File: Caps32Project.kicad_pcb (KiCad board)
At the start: 2 copper layers, 20 x 33 mm, 36 parts, among them J1 Ph 2.0, J2 Sh 1.0, P1 USB_C_Plug_USB2.0, Q1 AO3401A, U1 MPU-6050, U2 IP5306, U3 ESP32C3_SuperMini

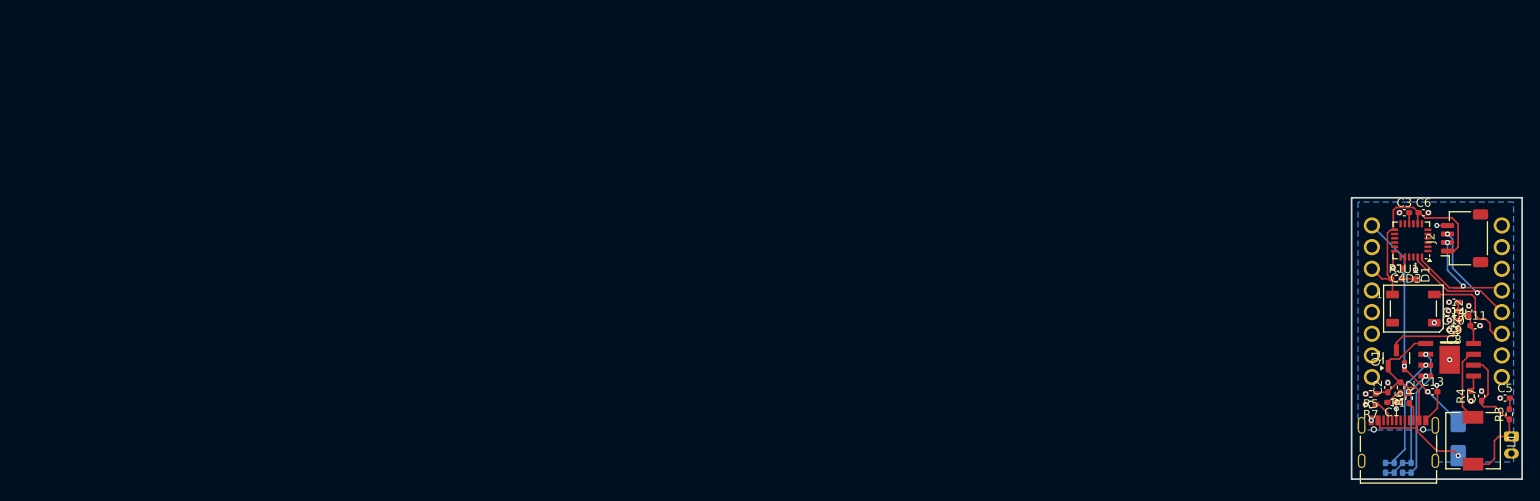
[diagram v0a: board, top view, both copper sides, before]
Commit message: Tweak
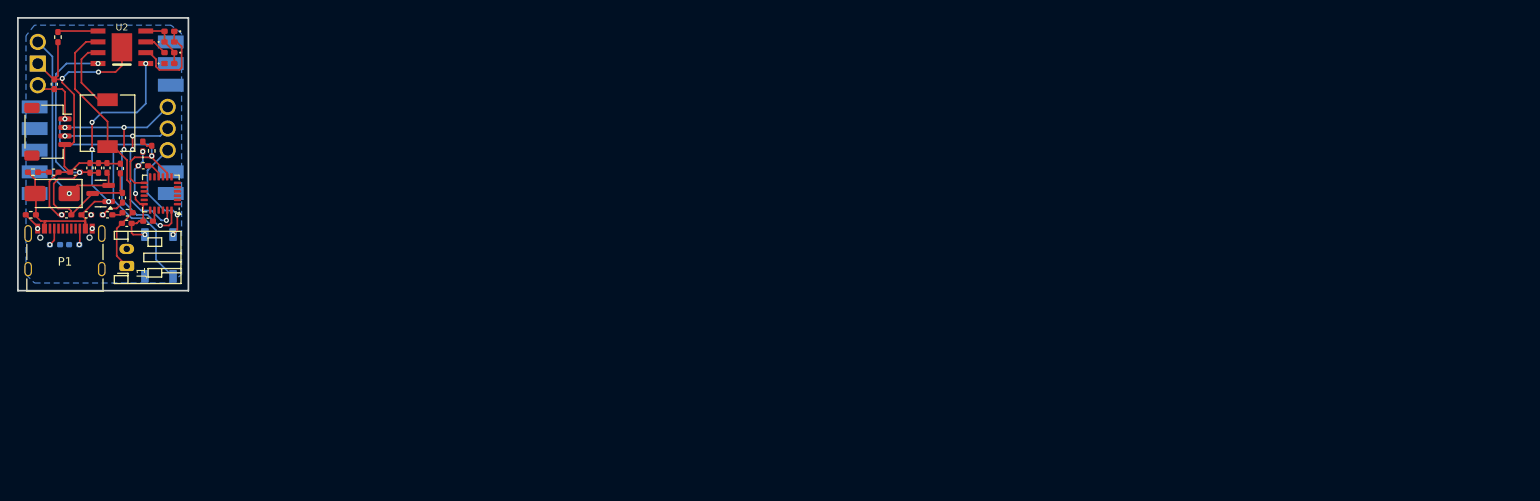
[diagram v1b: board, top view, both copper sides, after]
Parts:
- D2, D4, D5, D6, D7, J1: moved to F.Cu
- D3, R6, R7: moved to B.Cu
- U3: footprint Custom:ESP32C3_Supermini_THT -> Custom:Supermini_Custom
- moved R4 171.0 mm to (30.2, 27.7)
- moved D6 167.4 mm to (29.6, 46.0), turned to 180 degrees
- moved J2 166.7 mm to (29.1, 38.8), turned to -90 degrees
- moved C11 165.8 mm to (31.2, 48.5), turned to 180 degrees
- moved C5 165.3 mm to (36.1, 48.5)
- moved L1 164.5 mm to (36.1, 37.8)
- moved C12 164.3 mm to (32.2, 43.5), turned to 180 degrees
- moved R3 163.8 mm to (38.4, 48.2), turned to 180 degrees
- moved J1 163.7 mm to (38.3, 54.5), turned to 90 degrees
- moved R2 162.4 mm to (27.3, 43.5), turned to 0 degrees
- moved C6 161.3 mm to (29.8, 33.2), turned to 90 degrees
- moved C10 160.8 mm to (34.0, 43.0), turned to 90 degrees
- moved C7 160.2 mm to (38.3, 49.5), turned to 0 degrees
- moved C9 160.0 mm to (35.0, 43.0), turned to 90 degrees
- moved U2 160.0 mm to (37.8, 28.8), turned to 90 degrees
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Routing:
- net GND: track 10.7 -> 63.5 mm, vias 22 -> 11
- net +3V3: track 27.6 -> 51.1 mm, vias 0 -> 2
- net VCC: track 17.1 -> 39.6 mm, vias 0 -> 2
- net +BATT: track 19.4 -> 32.7 mm
- net SDA: track 18.3 -> 30.3 mm, vias 2 -> 4
- net Net-(D5-A): track 14.0 -> 2.72 mm, vias 1 -> 0
- net VBUS: track 30.6 -> 41.2 mm, vias 1 -> 4
- net Net-(D2-K): track 14.5 -> 6.47 mm, vias 1 -> 0
- net Net-(D2-A): track 16.1 -> 10.5 mm, vias 1 -> 0
- net SCL: track 21.2 -> 26.5 mm, vias 2 -> 4
- net Net-(U2-KEY): track 1.87 -> 4.75 mm
- net RGB: track 11.4 -> 13.1 mm, vias 0 -> 2
- net +5V: track 27.2 -> 25.9 mm, vias 2 -> 1
- net Net-(C1-Pad2): track 2.04 -> 1.27 mm
- net Net-(U1-REGOUT): track 1.30 -> 2.06 mm
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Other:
- board size 20 x 33 mm -> 20 x 32 mm

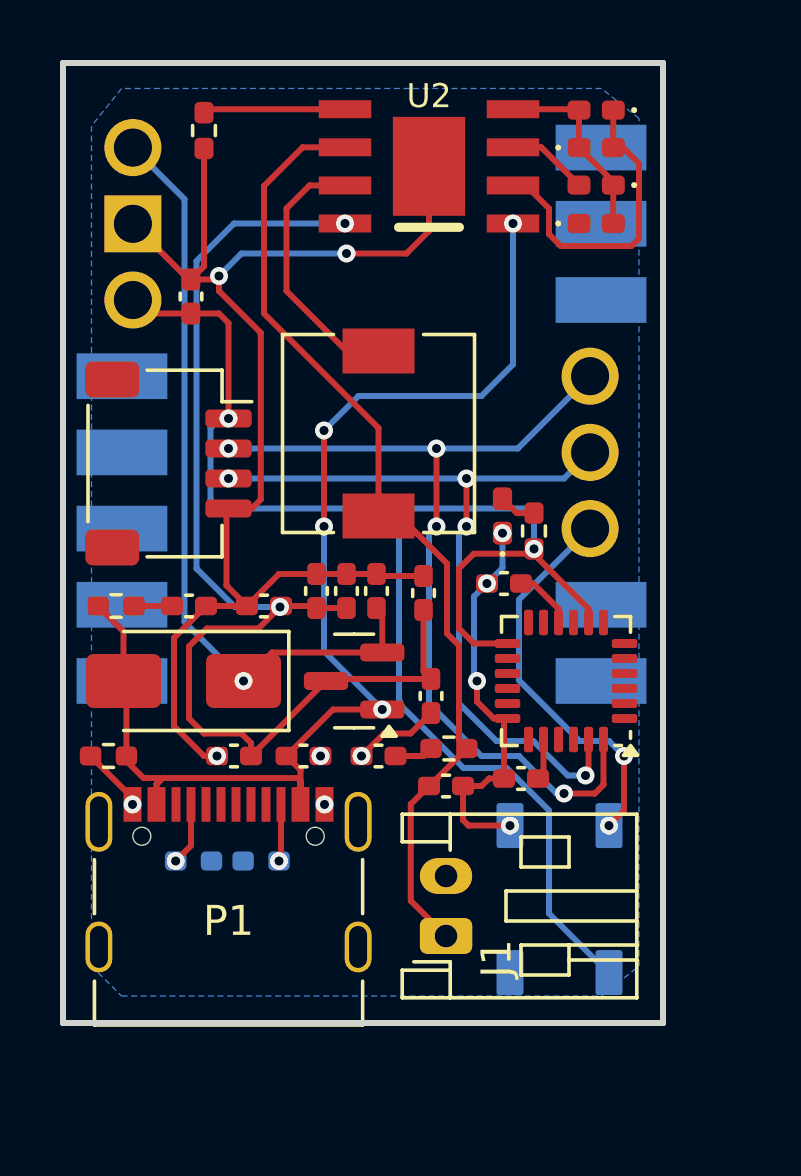
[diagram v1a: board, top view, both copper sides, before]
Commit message: Fixing
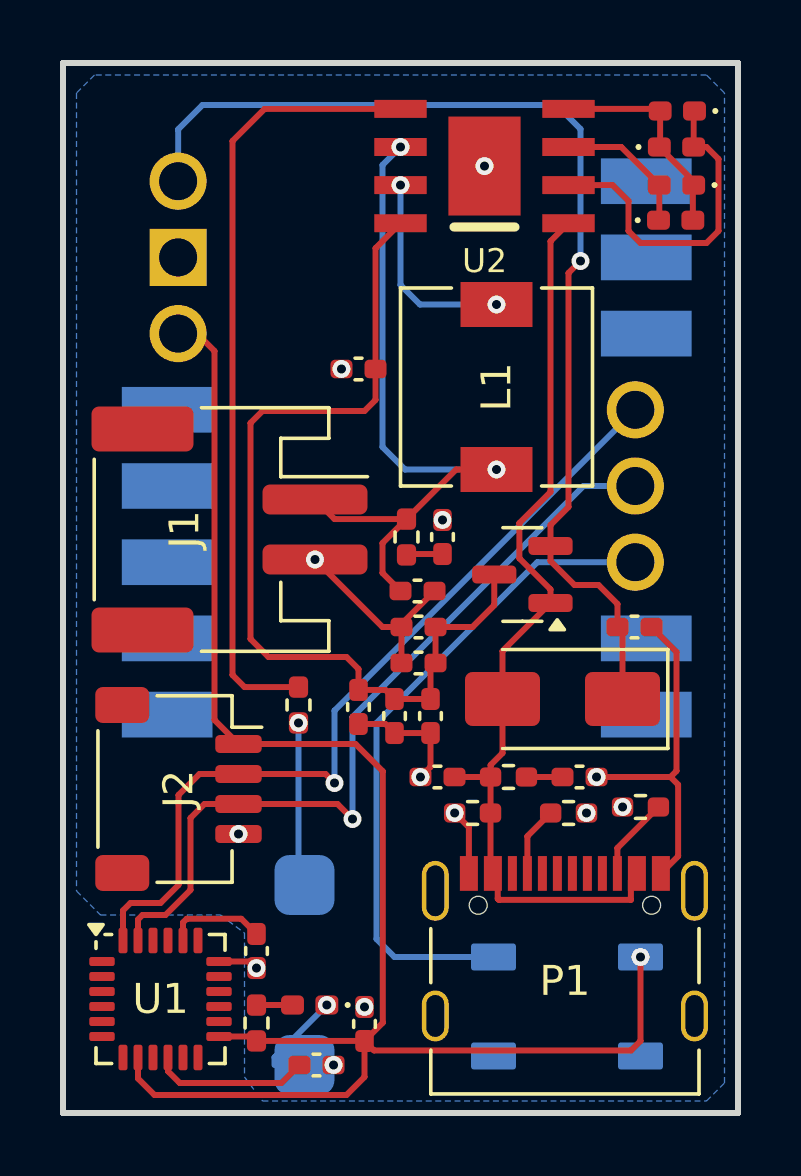
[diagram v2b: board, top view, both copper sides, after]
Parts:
- added SW1: SW_Push, Button_Switch_SMD:SW_Push_1TS009xxxx-xxxx-xxxx_6x6x5mm, B.Cu at (33.6, 55.8)
- J1: footprint Connector_JST:JST_PH_S2B-PH-K_1x02_P2.00mm_Horizontal -> Connector_JST:JST_PH_S2B-PH-SM4-TB_1x02-1MP_P2.00mm_Horizontal
- R6, R7: moved to F.Cu
- moved C6 24.9 mm to (35.6, 57.4)
- moved R4 19.4 mm to (33.4, 46.8)
- moved R1 18.8 mm to (32.0, 57.4)
- moved D1 17.5 mm to (33.8, 56.8), turned to 180 degrees
- moved C3 17.2 mm to (34.0, 58.8), turned to 180 degrees
- moved U1 17.2 mm to (28.8, 56.6), turned to 0 degrees
- moved J1 15.4 mm to (31.1, 41.0), turned to -90 degrees
- moved R2 14.3 mm to (40.4, 49.2)
- moved C1 14.2 mm to (42.8, 49.2)
- moved R6 12.8 mm to (44.8, 50.2)
- moved D6 12.6 mm to (42.2, 46.6)
- moved R7 12.6 mm to (42.4, 50.4)
- moved R5 12.3 mm to (39.2, 50.4)
- moved P1 11.4 mm to (42.3, 54.9)
- moved J2 10.9 mm to (29.4, 49.6)
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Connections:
- R4 pad 1: GND -> Net-(R4-Pad1)
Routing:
- net GND: track 63.5 -> 28.5 mm, vias 11 -> 14
- net Net-(U2-KEY): track 4.75 -> 26.2 mm
- net +5V: track 25.9 -> 36.7 mm
- net VBUS: track 41.2 -> 31.2 mm, vias 4 -> 0
- net RGB: track 13.1 -> 22.2 mm, vias 2 -> 0
- net VCC: track 39.6 -> 30.9 mm, vias 2 -> 0
- net +BATT: track 32.7 -> 24.3 mm, vias 0 -> 2
- net Net-(R4-Pad1): track 0.00 -> 5.49 mm, vias 0 -> 1
- net +3V3: track 51.1 -> 56.4 mm, vias 2 -> 1
- net Net-(U1-REGOUT): track 2.06 -> 5.25 mm
- net Net-(U2-SW): track 8.91 -> 6.80 mm, vias 0 -> 2
- net Net-(D5-A): track 2.72 -> 4.73 mm
- net Net-(U1-CPOUT): track 1.38 -> 3.31 mm
- net SDA: track 30.3 -> 28.4 mm, vias 4 -> 1
- net Net-(P1-CC2): track 1.91 -> 2.78 mm, vias 1 -> 0
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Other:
- board size 20 x 32 mm -> 22.5 x 35 mm
